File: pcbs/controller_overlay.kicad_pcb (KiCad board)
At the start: 2 copper layers, 22 x 62.8 mm, 2 parts

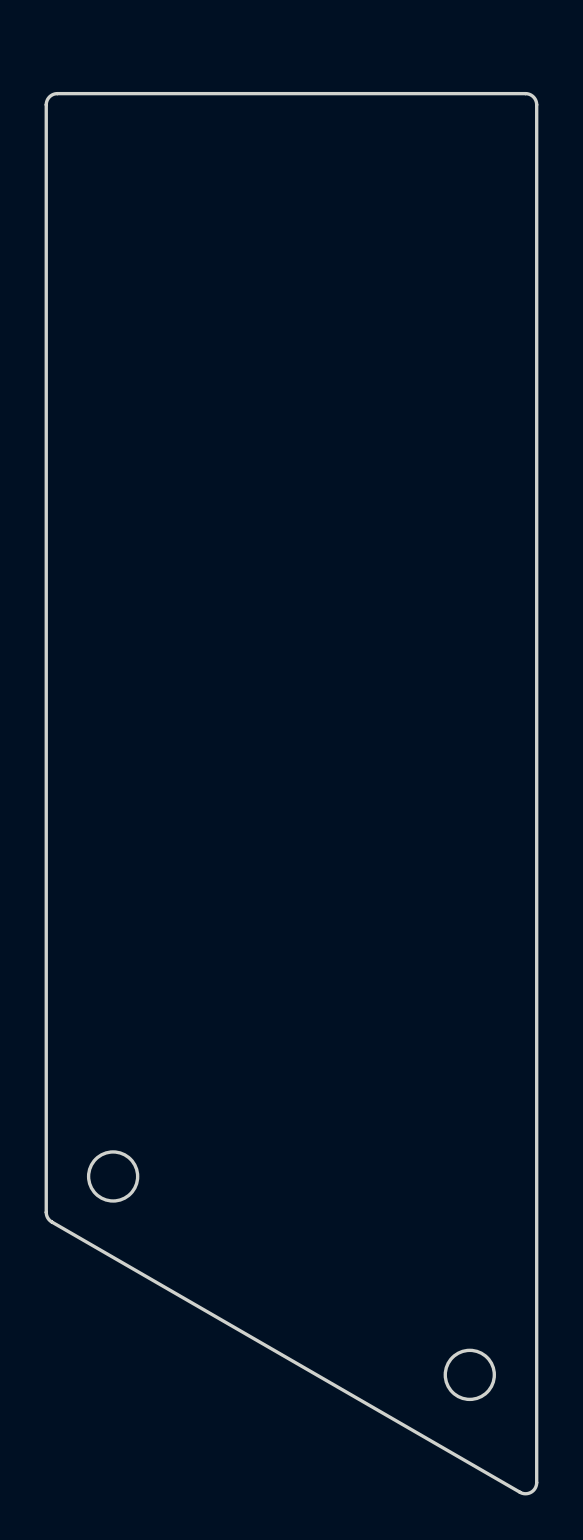
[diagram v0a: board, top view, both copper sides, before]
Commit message: staggero_change
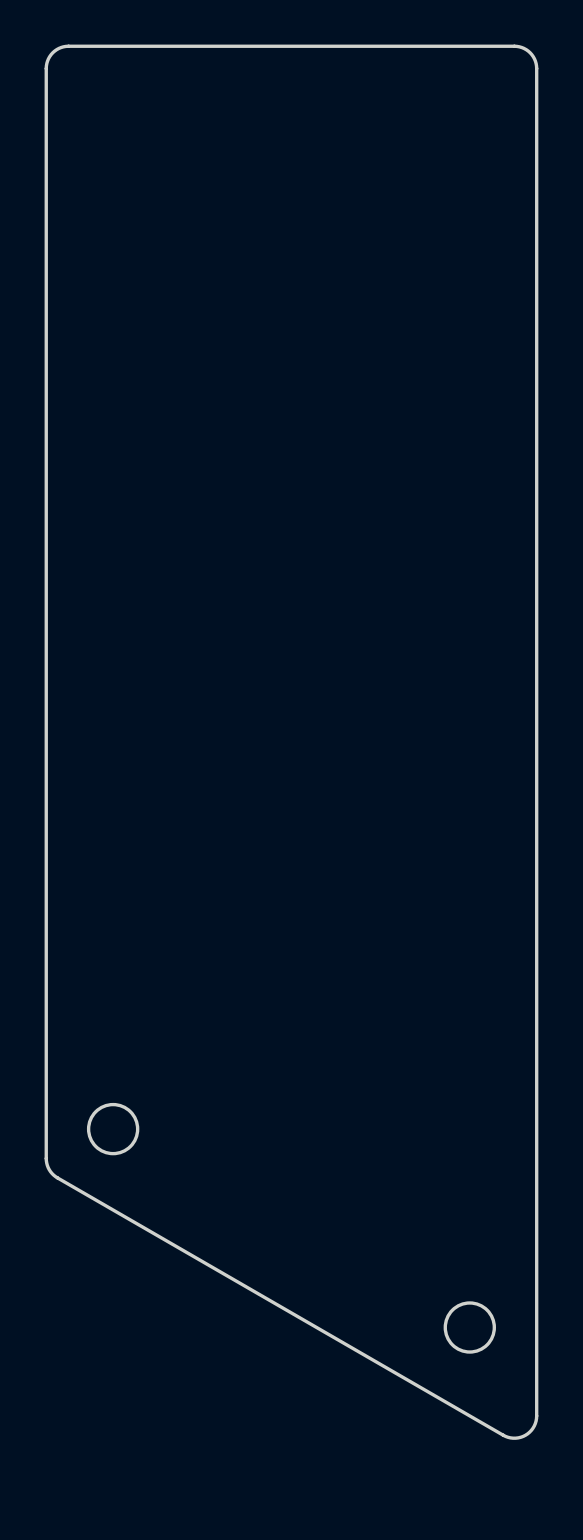
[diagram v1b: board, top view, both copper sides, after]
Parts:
- moved MH1 2.12 mm to (185.0, 105.6)
- moved MH2 2.12 mm to (201.0, 114.5)
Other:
- board size 22 x 62.8 mm -> 22 x 62.4 mm
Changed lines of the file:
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@@
 	(title_block
 		(title "controller_overlay")
-		(date "2024-11-30")
+		(date "2024-12-31")
 		(rev "0.2")
 		(company "ceoloide")
@@
 	(footprint "ceoloide:mounting_hole_npth"
 		(layer "F.Cu")
-		(at 185 107.7)
+		(at 185 105.575)
 		(property "Reference" "MH1"
 			(at 0 2.55 0)
@@
 	(footprint "ceoloide:mounting_hole_npth"
 		(layer "F.Cu")
-		(at 201 116.6)
+		(at 201 114.475)
 		(property "Reference" "MH2"
 			(at 0 2.55 0)
@@
 	)
 	(gr_line
-		(start 182.5 59.125)
-		(end 203.5 59.125)
+		(start 204 58)
+		(end 204 118.441813)
+		(stroke
+			(width 0.15)
+			(type default)
+		)
+		(layer "Edge.Cuts")
+	)
+	(gr_arc
+		(start 204 118.441813)
+		(mid 203.500058 119.308073)
+		(end 202.5 119.307838)
+		(stroke
+			(width 0.15)
+			(type default)
+		)
+		(layer "Edge.Cuts")
+	)
+	(gr_line
+		(start 183 57)
+		(end 203 57)
+		(stroke
+			(width 0.15)
+			(type default)
+		)
+		(layer "Edge.Cuts")
+	)
+	(gr_arc
+		(start 182.5 107.760833)
+		(mid 182.133972 107.394808)
+		(end 182 106.894808)
+		(stroke
+			(width 0.15)
+			(type default)
+		)
+		(layer "Edge.Cuts")
+	)
+	(gr_arc
+		(start 203 57)
+		(mid 203.707107 57.292893)
+		(end 204 58)
+		(stroke
+			(width 0.15)
+			(type default)
+		)
+		(layer "Edge.Cuts")
+	)
+	(gr_arc
+		(start 182 58)
+		(mid 182.292893 57.292893)
+		(end 183 57)
+		(stroke
+			(width 0.15)
+			(type default)
+		)
+		(layer "Edge.Cuts")
+	)
+	(gr_line
+		(start 202.5 119.307838)
+		(end 182.5 107.760833)
 		(stroke
 			(width 0.15)
@@
 	)
 	(gr_circle
-		(center 201 116.6)
-		(end 202.1 116.6)
+		(center 201 114.475)
+		(end 202.1 114.475)
 		(stroke
 			(width 0.15)
@@
 	)
 	(gr_circle
-		(center 185 107.7)
-		(end 186.1 107.7)
+		(center 185 105.575)
+		(end 186.1 105.575)
 		(stroke
 			(width 0.15)
@@
 		(layer "Edge.Cuts")
 	)
-	(gr_arc
-		(start 203.5 59.125)
-		(mid 203.853553 59.271447)
-		(end 204 59.625)
-		(stroke
-			(width 0.15)
-			(type default)
-		)
-		(layer "Edge.Cuts")
-	)
-	(gr_line
-		(start 182 109.308483)
-		(end 182 59.625)
-		(stroke
-			(width 0.15)
-			(type default)
-		)
-		(layer "Edge.Cuts")
-	)
-	(gr_line
-		(start 203.25 121.865851)
-		(end 182.25 109.741495)
-		(stroke
-			(width 0.15)
-			(type default)
-		)
-		(layer "Edge.Cuts")
-	)
-	(gr_line
-		(start 204 59.625)
-		(end 204 121.432838)
-		(stroke
-			(width 0.15)
-			(type default)
-		)
-		(layer "Edge.Cuts")
-	)
-	(gr_arc
-		(start 204 121.432838)
-		(mid 203.750061 121.866098)
-		(end 203.25 121.865851)
-		(stroke
-			(width 0.15)
-			(type default)
-		)
-		(layer "Edge.Cuts")
-	)
-	(gr_arc
-		(start 182.25 109.741495)
-		(mid 182.066994 109.558481)
-		(end 182 109.308483)
-		(stroke
-			(width 0.15)
-			(type default)
-		)
-		(layer "Edge.Cuts")
-	)
-	(gr_arc
-		(start 182 59.625)
-		(mid 182.146447 59.271447)
-		(end 182.5 59.125)
-		(stroke
-			(width 0.15)
+	(gr_line
+		(start 182 106.894808)
+		(end 182 58)
+		(stroke
+			(width 0.15)
